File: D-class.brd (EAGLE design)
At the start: 65 parts, among them IC1 TPA3118D2, IC2 78L12, IC3 7812

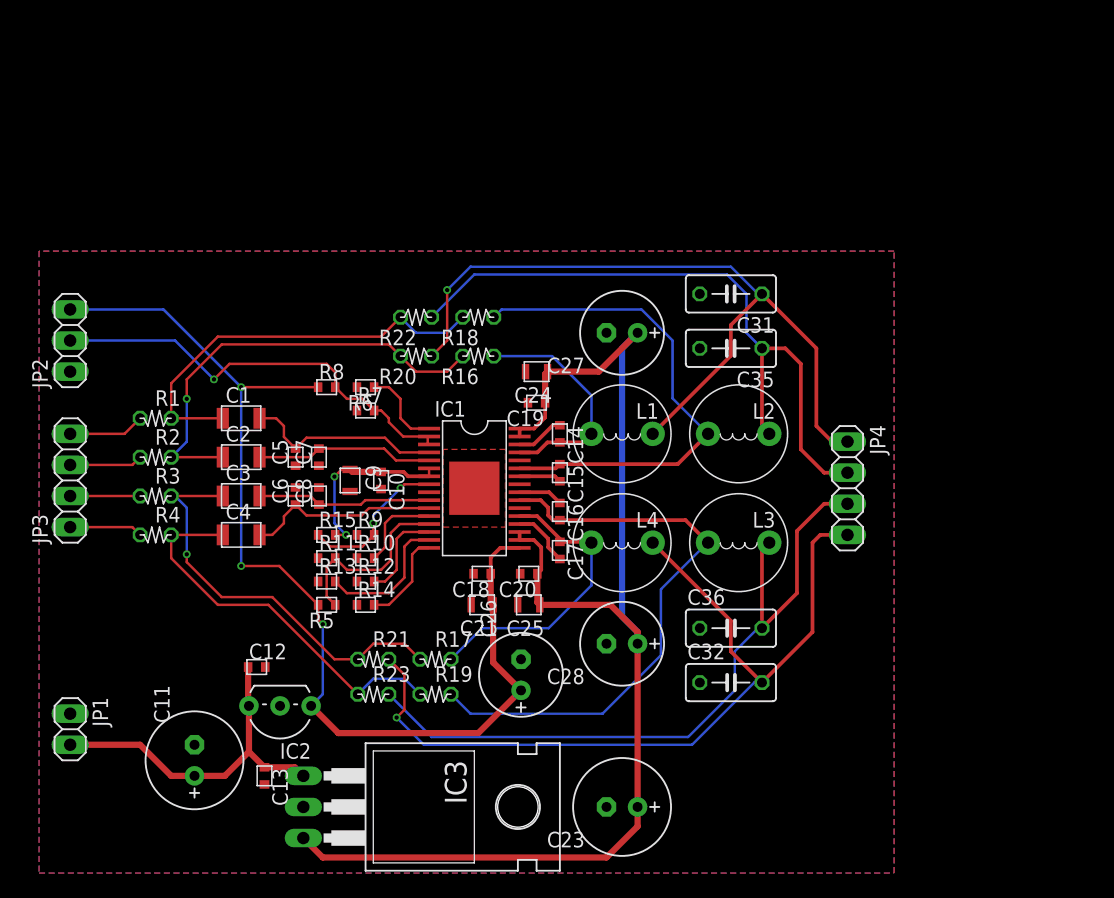
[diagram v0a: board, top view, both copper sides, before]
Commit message: 後はシルクのみ
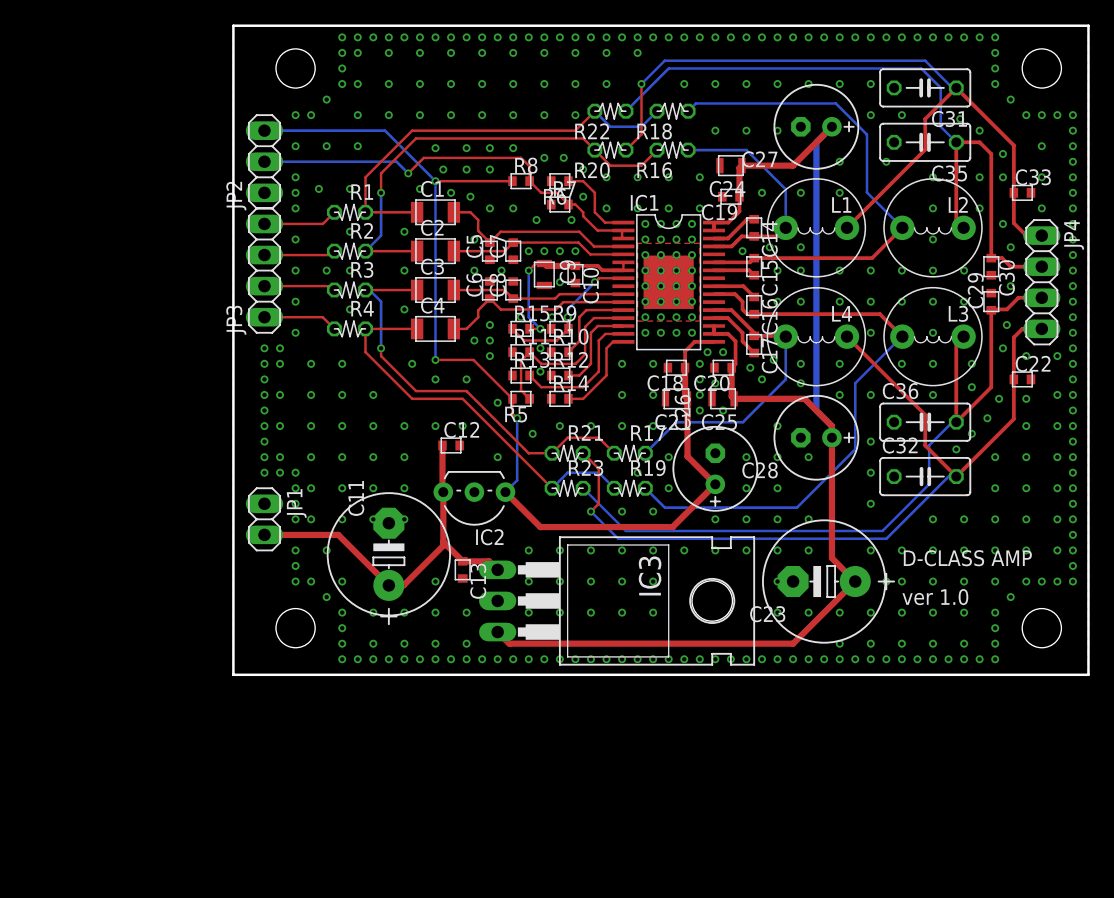
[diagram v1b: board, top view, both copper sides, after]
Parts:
- added C22, C29, C30, C33: 100p, my_rcl:1608
- added HOLE1, HOLE2, HOLE3, HOLE4: HOLE_3.2, Document_Robotech:HOLE_3.2
- C11, C23: device my_rcl:E2,5-8 -> my_rcl:E5-10
- moved C23 24.7 mm to (48.3, 7.62)
- moved C12 24.1 mm to (17.8, 18.7)
- moved IC2 23.6 mm to (19.7, 14.9)
- moved JP1 23.4 mm to (2.54, 12.7)
- moved JP3 23.4 mm to (2.54, 33.0)
- moved C13 23.4 mm to (18.7, 8.57)
- moved C1 23.1 mm to (16.5, 37.8)
- moved C10 23.1 mm to (27.9, 32.7)
- moved C14 23.1 mm to (42.5, 36.5)
- moved C2 23.1 mm to (16.5, 34.6)
- moved C20 23.1 mm to (40.0, 25.1)
- moved C25 23.1 mm to (40.0, 22.5)
- moved C3 23.1 mm to (16.5, 31.4)
- moved C31 23.1 mm to (56.5, 47.9)
- moved C4 23.1 mm to (16.5, 28.3)
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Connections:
- net GND: now also C22.2, C29.2, C30.2, C33.2
- net N$25: now also C29.1
- net N$26: now also C22.1
- net N$27: now also C30.1
- net N$28: now also C33.1
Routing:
- net VCC: track 28.7 -> 31.3 mm
- net AVCC: track 88.0 -> 86.7 mm
- net SLEEP: track 35.2 -> 34.3 mm
- net N$27: track 55.3 -> 56.2 mm
- net N$25: track 58.9 -> 59.6 mm
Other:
- board outline added: 69.8 x 53 mm
- board text added: "D-CLASS AMP"
- board text added: "ver 1.0"
